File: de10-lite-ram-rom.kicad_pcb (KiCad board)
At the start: 2 copper layers, 52.1 x 33 mm, 8 parts, among them J6 DE10-Lite GPIO, U1 AS6C4008A-55ZIN, U2 SST39LF040

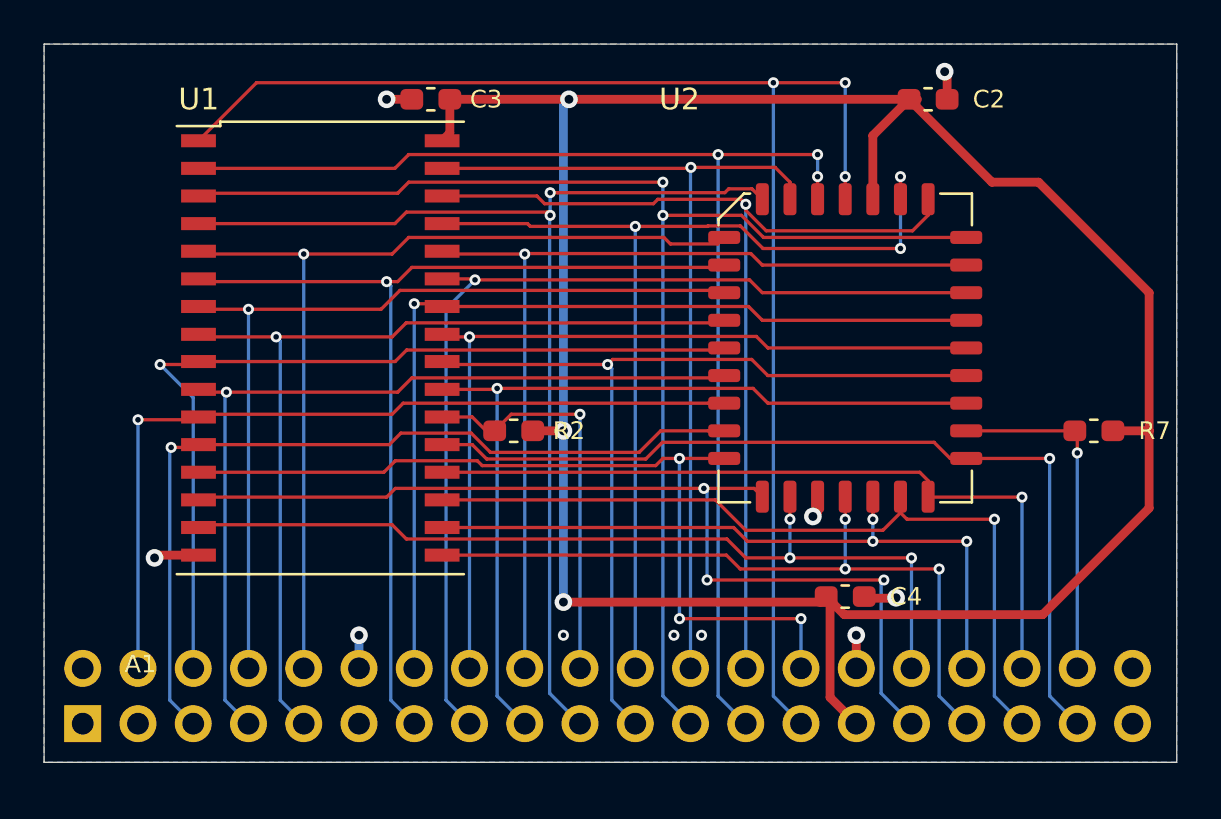
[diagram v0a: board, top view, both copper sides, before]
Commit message: Final version
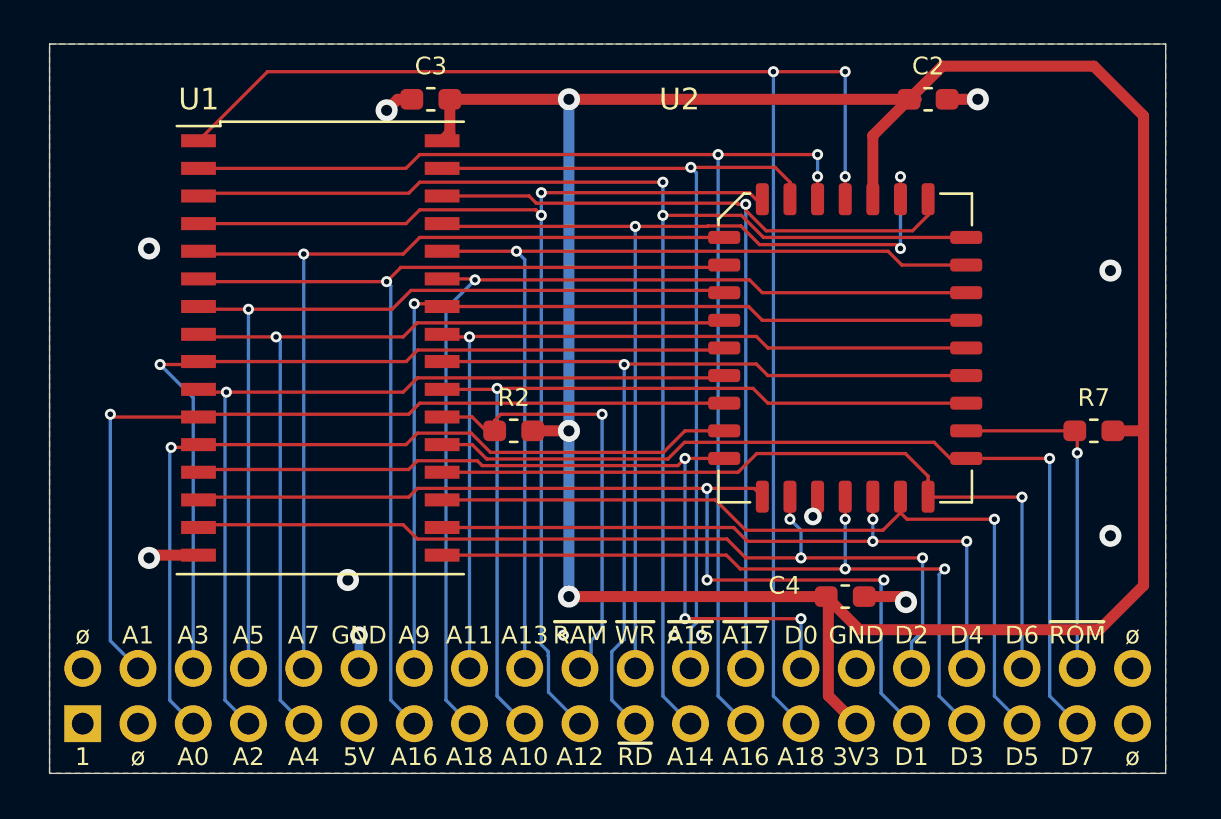
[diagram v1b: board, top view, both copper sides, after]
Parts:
- removed J6: DE10-Lite GPIO, Connector_PinSocket_2.54mm:PinSocket_2x20_P2.54mm_Vertical
- added G***: LOGO, Logos:asian_tiger, F.Cu at (154.7, 98.9)
- added J1: DE10-Lite_GPIO_Header, Connector_PinSocket_2.54mm:PinSocket_2x20_P2.54mm_Horizontal, F.Cu at (131.3, 115.1)
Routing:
- net VCC: track 115.6 -> 123.9 mm
- net /A1: track 38.7 -> 40.7 mm
- net /RAM_~CE: track 18.6 -> 20.3 mm
- net /D6: track 35.4 -> 37.0 mm
- net /A18: track 66.2 -> 67.4 mm
- net /D2: track 41.1 -> 42.3 mm
- net GND: track 10.1 -> 9.76 mm, vias 10 -> 13
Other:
- board size 52.1 x 33 mm -> 51.3 x 33.5 mm
- net class Power: trace_width 0.4064 -> 0.508; via_dia 0.8128 -> 1.016; via_drill 0.4064 -> 0.508
- board text added: "1"
- board text added: "3V3"
- board text added: "5V"
- board text added: "A0"
- board text added: "A10"
- board text added: "A11"
- board text added: "A12"
- board text added: "A13"
- board text added: "A14"
- board text added: "A16"
- board text added: "A18"
- board text added: "A2"
- board text added: "A3"
- board text added: "A4"
- board text added: "A5"
- board text added: "A7"
- board text added: "A9"
- board text added: "D0"
- board text added: "D1"
- board text added: "D2"
- board text added: "D3"
- board text added: "D4"
- board text added: "D5"
- board text added: "D6"
- board text added: "D7"
- board text added: "DE10-Lite 512K SRAM/Flash ROM Board version 1.0 by Hyiger Designs"
- board text added: "GND"
- board text added: "~A15"
- board text added: "~A17"
- board text added: "~RAM"
- board text added: "~RD"
- board text added: "~ROM"
- board text added: "~WR"
- board text added: "ø"
